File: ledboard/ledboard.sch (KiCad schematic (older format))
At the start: 49 parts, among them J1 LEFT, J2 PWR_L, J3 RIGHT, J4 PWR_R, J5 Conn_01x03_Male, J6 Conn_01x02_Male, J7 Conn_02x20_Odd_Even, J8 Conn_01x02_Shielded, M1 MPMOS, U1 AL8860, U2 AL8860, U3 LM22676MR-5

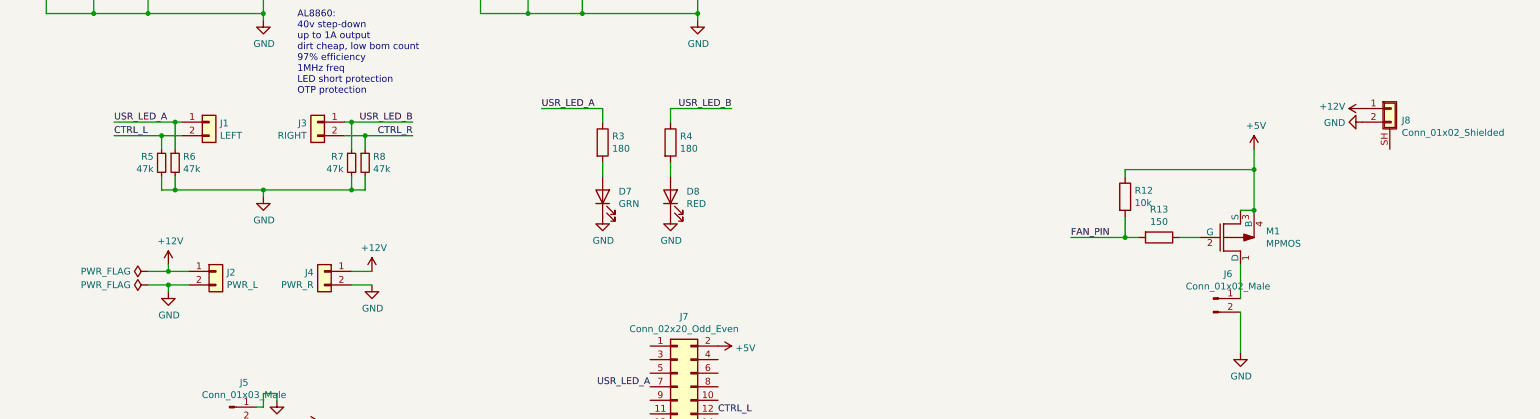
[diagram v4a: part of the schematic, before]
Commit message: power soket
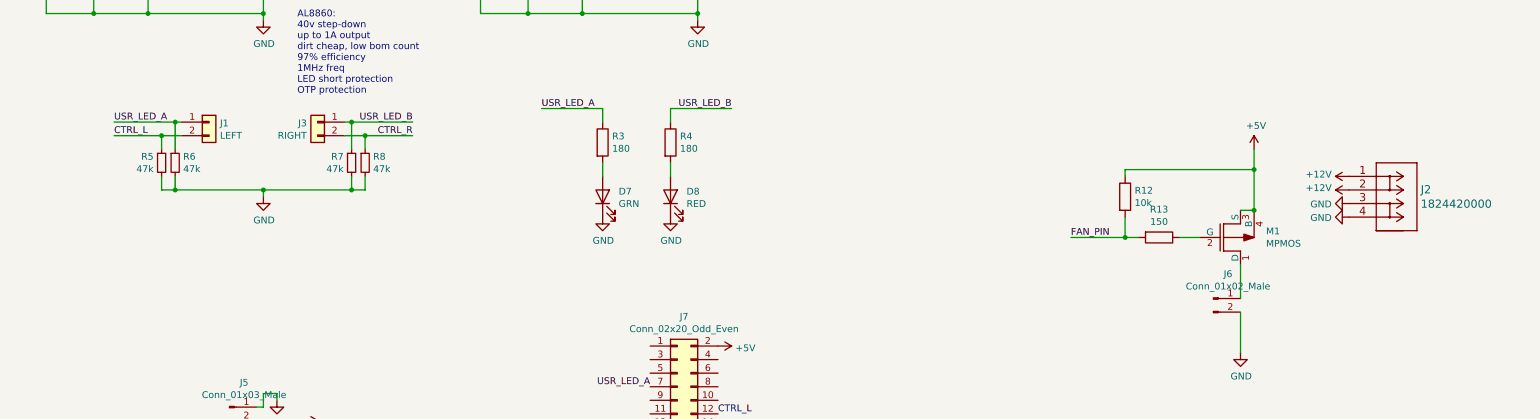
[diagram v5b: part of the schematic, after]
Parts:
- removed J2: PWR_L, ledboard:PinHeader_1x02_P2.54mm_Vertical_RoundRect, symbol Connector_Generic:Conn_01x02
- removed J4: PWR_R, ledboard:PinHeader_1x02_P2.54mm_Vertical_RoundRect, symbol Connector_Generic:Conn_01x02
- removed J8: Conn_01x02_Shielded, Connector:TE_282837-2, symbol Connector_Generic_Shielded:Conn_01x02_Shielded
- added J2: 1824420000, footprints:1824420000, symbol 2020-12-27_12-53-24:1824420000
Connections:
- net +12V: now also J2.1, J2.2
- net GND: now also J2.3, J2.4
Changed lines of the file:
@@
 Text Label 3450 3800 2    50   ~ 0
 CTRL_R
-$Comp
-L power:GND #PWR06
-U 1 1 5E99C0D4
-P 3150 4900
-F 0 "#PWR06" H 3150 4650 50  0001 C CNN
-F 1 "GND" H 3155 4727 50  0000 C CNN
-F 2 "" H 3150 4900 50  0001 C CNN
-F 3 "" H 3150 4900 50  0001 C CNN
-	1    3150 4900
-	1    0    0    -1
-$EndComp
-$Comp
-L power:GND #PWR03
-U 1 1 5E99C601
-P 1650 4950
-F 0 "#PWR03" H 1650 4700 50  0001 C CNN
-F 1 "GND" H 1655 4777 50  0000 C CNN
-F 2 "" H 1650 4950 50  0001 C CNN
-F 3 "" H 1650 4950 50  0001 C CNN
-	1    1650 4950
-	1    0    0    -1
-$EndComp
-Wire Wire Line
-	3000 4800 3150 4800
-Wire Wire Line
-	3150 4900 3000 4900
 Wire Wire Line
 	1650 2600 1950 2600
@@
 	5650 1250 6650 1250
 $Comp
-L power:PWR_FLAG #FLG0101
-U 1 1 68FB9579
-P 1500 4800
-F 0 "#FLG0101" H 1500 4875 50  0001 C CNN
-F 1 "PWR_FLAG" V 1500 4927 50  0000 L CNN
-F 2 "" H 1500 4800 50  0001 C CNN
-F 3 "~" H 1500 4800 50  0001 C CNN
-	1    1500 4800
-	0    -1   -1   0
-$EndComp
-$Comp
-L power:PWR_FLAG #FLG0102
-U 1 1 68FB9AC1
-P 1500 4900
-F 0 "#FLG0102" H 1500 4975 50  0001 C CNN
-F 1 "PWR_FLAG" V 1500 5027 50  0000 L CNN
-F 2 "" H 1500 4900 50  0001 C CNN
-F 3 "~" H 1500 4900 50  0001 C CNN
-	1    1500 4900
-	0    -1   -1   0
-$EndComp
-$Comp
 L Connector_Generic:Conn_01x02 J3
 U 1 1 68FC2202
@@
 $EndComp
 $Comp
-L Connector_Generic:Conn_01x02 J2
-U 1 1 68FC3D82
-P 2000 4800
-F 0 "J2" H 2080 4792 50  0000 L CNN
-F 1 "PWR_L" H 2080 4701 50  0000 L CNN
-F 2 "ledboard:PinHeader_1x02_P2.54mm_Vertical_RoundRect" H 2000 4800 50  0001 C CNN
-F 3 "~" H 2000 4800 50  0001 C CNN
-F 4 "MTP125-1102S1" H 2000 4800 50  0001 C CNN "P/N"
-F 5 "C358684" H 2000 4800 50  0001 C CNN "LCSC"
-F 6 "" H 2000 4800 50  0001 C CNN "Digikey"
-F 7 "No" H 2000 4800 50  0001 C CNN "Generic OK"
-	1    2000 4800
-	1    0    0    -1
-$EndComp
-$Comp
 L Device:L L2
 U 1 1 68FC6A75
@@
 Wire Wire Line
 	3000 4100 3000 4200
-Wire Wire Line
-	1500 4800 1650 4800
-Wire Wire Line
-	1500 4900 1650 4900
-Wire Wire Line
-	1650 4950 1650 4900
-Connection ~ 1650 4900
-Wire Wire Line
-	1650 4900 1800 4900
-Wire Wire Line
-	1650 4800 1650 4750
-Connection ~ 1650 4800
-Wire Wire Line
-	1650 4800 1800 4800
 $Comp
 L Device:D_Schottky D4
@@
 CTRL_L
 $Comp
-L Connector_Generic:Conn_01x02 J4
-U 1 1 68FC5398
-P 2800 4800
-F 0 "J4" H 2880 4792 50  0000 L CNN
-F 1 "PWR_R" H 2880 4701 50  0000 L CNN
-F 2 "ledboard:PinHeader_1x02_P2.54mm_Vertical_RoundRect" H 2800 4800 50  0001 C CNN
-F 3 "~" H 2800 4800 50  0001 C CNN
-F 4 "MTP125-1102S1" H 2800 4800 50  0001 C CNN "P/N"
-F 5 "C358684" H 2800 4800 50  0001 C CNN "LCSC"
-F 6 "" H 2800 4800 50  0001 C CNN "Digikey"
-F 7 "No" H 2800 4800 50  0001 C CNN "Generic OK"
-	1    2800 4800
-	-1   0    0    -1
-$EndComp
-$Comp
 L Connector:Conn_01x03_Male J5
 U 1 1 5F67D78E
@@
 Wire Wire Line
 	9550 5100 9550 5400
-$Comp
-L Connector_Generic_Shielded:Conn_01x02_Shielded J8
-U 1 1 5F990056
-P 10650 3600
-F 0 "J8" H 10738 3513 50  0000 L CNN
-F 1 "Conn_01x02_Shielded" H 10738 3422 50  0000 L CNN
-F 2 "Connector:TE_282837-2" H 10650 3600 50  0001 C CNN
-F 3 "~" H 10650 3600 50  0001 C CNN
-F 4 "282837-2" H 10650 3600 50  0001 C CNN "P/N"
-	1    10650 3600
-	1    0    0    -1
-$EndComp
 Wire Wire Line
 	7550 1400 7550 1650
@@
 L power:+12V #PWR0102
 U 1 1 5F9E5194
-P 10450 3600
-F 0 "#PWR0102" H 10450 3450 50  0001 C CNN
-F 1 "+12V" V 10465 3728 50  0000 L CNN
-F 2 "" H 10450 3600 50  0001 C CNN
-F 3 "" H 10450 3600 50  0001 C CNN
-	1    10450 3600
+P 10350 4100
+F 0 "#PWR0102" H 10350 3950 50  0001 C CNN
+F 1 "+12V" V 10365 4228 50  0000 L CNN
+F 2 "" H 10350 4100 50  0001 C CNN
+F 3 "" H 10350 4100 50  0001 C CNN
+	1    10350 4100
 	0    -1   -1   0
 $EndComp
@@
 $EndComp
 $Comp
-L power:+12V #PWR0108
-U 1 1 5FA22F73
-P 1650 4750
-F 0 "#PWR0108" H 1650 4600 50  0001 C CNN
-F 1 "+12V" H 1665 4923 50  0000 C CNN
-F 2 "" H 1650 4750 50  0001 C CNN
-F 3 "" H 1650 4750 50  0001 C CNN
-	1    1650 4750
-	1    0    0    -1
-$EndComp
-$Comp
-L power:+12V #PWR0109
-U 1 1 5FA235FC
-P 3150 4800
-F 0 "#PWR0109" H 3150 4650 50  0001 C CNN
-F 1 "+12V" H 3165 4973 50  0000 C CNN
-F 2 "" H 3150 4800 50  0001 C CNN
-F 3 "" H 3150 4800 50  0001 C CNN
-	1    3150 4800
-	1    0    0    -1
-$EndComp
-$Comp
 L power:+5V #PWR0110
 U 1 1 5FA33C77
@@
 L power:GND #PWR0114
 U 1 1 5FDA13DE
-P 10450 3700
-F 0 "#PWR0114" H 10450 3450 50  0001 C CNN
-F 1 "GND" V 10455 3572 50  0000 R CNN
-F 2 "" H 10450 3700 50  0001 C CNN
-F 3 "" H 10450 3700 50  0001 C CNN
-	1    10450 3700
+P 10350 4300
+F 0 "#PWR0114" H 10350 4050 50  0001 C CNN
+F 1 "GND" V 10355 4172 50  0000 R CNN
+F 2 "" H 10350 4300 50  0001 C CNN
+F 3 "" H 10350 4300 50  0001 C CNN
+	1    10350 4300
 	0    1    1    0
 $EndComp
@@
 	1    0    0    -1
 $EndComp
+$Comp
+L 2020-12-27_12-53-24:1824420000 J2
+U 1 1 5FE94EC7
+P 10350 4100
+F 0 "J2" H 10878 4003 60  0000 L CNN
+F 1 "1824420000" H 10878 3897 60  0000 L CNN
+F 2 "footprints:1824420000" H 10750 3840 60  0001 C CNN
+F 3 "" H 10350 4100 60  0000 C CNN
+	1    10350 4100
+	1    0    0    -1
+$EndComp
+$Comp
+L power:+12V #PWR0108
+U 1 1 5FEBFC3B
+P 10350 4200
+F 0 "#PWR0108" H 10350 4050 50  0001 C CNN
+F 1 "+12V" V 10365 4328 50  0000 L CNN
+F 2 "" H 10350 4200 50  0001 C CNN
+F 3 "" H 10350 4200 50  0001 C CNN
+	1    10350 4200
+	0    -1   -1   0
+$EndComp
+$Comp
+L power:GND #PWR0109
+U 1 1 5FECD213
+P 10350 4400
+F 0 "#PWR0109" H 10350 4150 50  0001 C CNN
+F 1 "GND" V 10355 4272 50  0000 R CNN
+F 2 "" H 10350 4400 50  0001 C CNN
+F 3 "" H 10350 4400 50  0001 C CNN
+	1    10350 4400
+	0    1    1    0
+$EndComp
 $EndSCHEMATC
